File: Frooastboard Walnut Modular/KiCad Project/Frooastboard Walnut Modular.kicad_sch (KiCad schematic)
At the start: 88 parts, among them J1 SW Interface, J2 Conn_01x16, J3 Conn_01x06, J4 Conn_01x06, J5 Conn_01x10, J6 Conn_01x12, J7 Conn_01x04, U1 RP2040, U2 SPX3819M5-L-3-3, U3 W25Q32JVZP, U4 nRF8001, U5 IS31FL3733-QF, U6 FS312F-G, U7 FS8205, U8 IP2312, Y1 32.768kHz, Y2 16MHz, Y3 12MHz

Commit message: stuff
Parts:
- removed BT1: Battery_Cell, TestPoint:TestPoint_2Pads_Pitch5.08mm_Drill1.3mm, symbol Device:Battery_Cell
- removed C1, C2, C4: 100n, Capacitor_SMD:C_0402_1005Metric, symbol Device:C_Small
- removed C10, C11: 12p, Capacitor_SMD:C_0402_1005Metric, symbol Device:C_Small
- removed C12: 1.8p, Capacitor_SMD:C_0402_1005Metric, symbol Device:C_Small
- removed C13: 1.2p, Capacitor_SMD:C_0402_1005Metric, symbol Device:C_Small
- removed C29: 10n, Capacitor_SMD:C_0805_2012Metric, symbol Device:C_Small
- removed C3: 1n, Capacitor_SMD:C_0402_1005Metric, symbol Device:C_Small
- removed C30, C36: 22u, Capacitor_SMD:C_0805_2012Metric, symbol Device:C
- removed C31: 10u, Capacitor_SMD:C_0805_2012Metric, symbol Device:C_Small
- removed C32: 100n, Capacitor_SMD:C_0805_2012Metric, symbol Device:C_Small
- removed C37: 10u, Capacitor_SMD:C_0805_2012Metric, symbol Device:C
- removed C5: 33n, Capacitor_SMD:C_0402_1005Metric, symbol Device:C_Small
- removed C6, C7: 15p, Capacitor_SMD:C_0402_1005Metric, symbol Device:C_Small
- removed C8: 2.2n, Capacitor_SMD:C_0402_1005Metric, symbol Device:C_Small
- removed C9: Not Mounted, Capacitor_SMD:C_0402_1005Metric, symbol Device:C_Small
- removed D1: GREEN, LED_SMD:LED_0805_2012Metric, symbol Device:LED
- removed D2: RED, LED_SMD:LED_0805_2012Metric, symbol Device:LED
- removed L1: 5.6nH, Inductor_SMD:L_0402_1005Metric, symbol Device:L_Small
- removed L2: 8.2nH, Inductor_SMD:L_0402_1005Metric, symbol Device:L_Small
- removed L3: 3.9nH, Inductor_SMD:L_0402_1005Metric, symbol Device:L_Small
- removed L4: 1uH, Inductor_SMD:L_6.3x6.3_H3, symbol Device:L
- removed R1: 10k, Resistor_SMD:R_0805_2012Metric, symbol Device:R_Small
- removed R10: 2k, Resistor_SMD:R_0805_2012Metric, symbol Device:R
- removed R12: 0k5, Resistor_SMD:R_0805_2012Metric, symbol Device:R
- removed R13, R14: 1M, Resistor_SMD:R_0805_2012Metric, symbol Device:R_Small
- removed R15, R16: 0k1, Resistor_SMD:R_0805_2012Metric, symbol Device:R
- removed R17, R20: NC, Resistor_SMD:R_0805_2012Metric, symbol Device:R
- removed R18: 51k, Resistor_SMD:R_0805_2012Metric, symbol Device:R
- removed R19: 1k, Resistor_SMD:R_0805_2012Metric, symbol Device:R
- removed R2: 22k, Resistor_SMD:R_0805_2012Metric, symbol Device:R_Small
- removed TP1: NRF_TXD, TestPoint:TestPoint_Pad_D1.5mm, symbol Connector:TestPoint
- removed TP2: NRF_RXD, TestPoint:TestPoint_Pad_D1.5mm, symbol Connector:TestPoint
- removed TP3: NRF_RESET, TestPoint:TestPoint_Pad_D1.5mm, symbol Connector:TestPoint
- removed TP4: NRF_IREF, TestPoint:TestPoint_Pad_D1.5mm, symbol Connector:TestPoint
- removed U2: SPX3819M5-L-3-3, Package_TO_SOT_SMD:SOT-23-5, symbol Regulator_Linear:SPX3819M5-L-3-3
- removed U4: nRF8001, Package_DFN_QFN:QFN-32-1EP_5x5mm_P0.5mm_EP3.45x3.45mm, symbol RF_Bluetooth:nRF8001
- removed U6: FS312F-G, Package_TO_SOT_SMD:SOT-23-6, symbol Frooastboard Symbols:FS312F-G
- removed U7: FS8205, Package_TO_SOT_SMD:SOT-23-6, symbol Frooastboard Symbols:FS8205
- removed U8: IP2312, Package_SO:SOIC-8-1EP_3.9x4.9mm_P1.27mm_EP2.41x3.3mm, symbol Frooastboard Symbols:IP2312
- removed Y1: 32.768kHz, Crystal:Crystal_SMD_EuroQuartz_EQ161-2Pin_3.2x1.5mm, symbol Device:Crystal_Small
- removed Y2: 16MHz, Crystal:Crystal_SMD_3225-4Pin_3.2x2.5mm, symbol Device:Crystal_GND24_Small
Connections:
- no-connect marks 6 -> 3
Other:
- note removed: "NC for 2.1A"
- note removed: "NC for 4.2V"
- moved on the sheet: C28, C33, C34, C35, J2, J3, J4, R11, R6, R7, U5

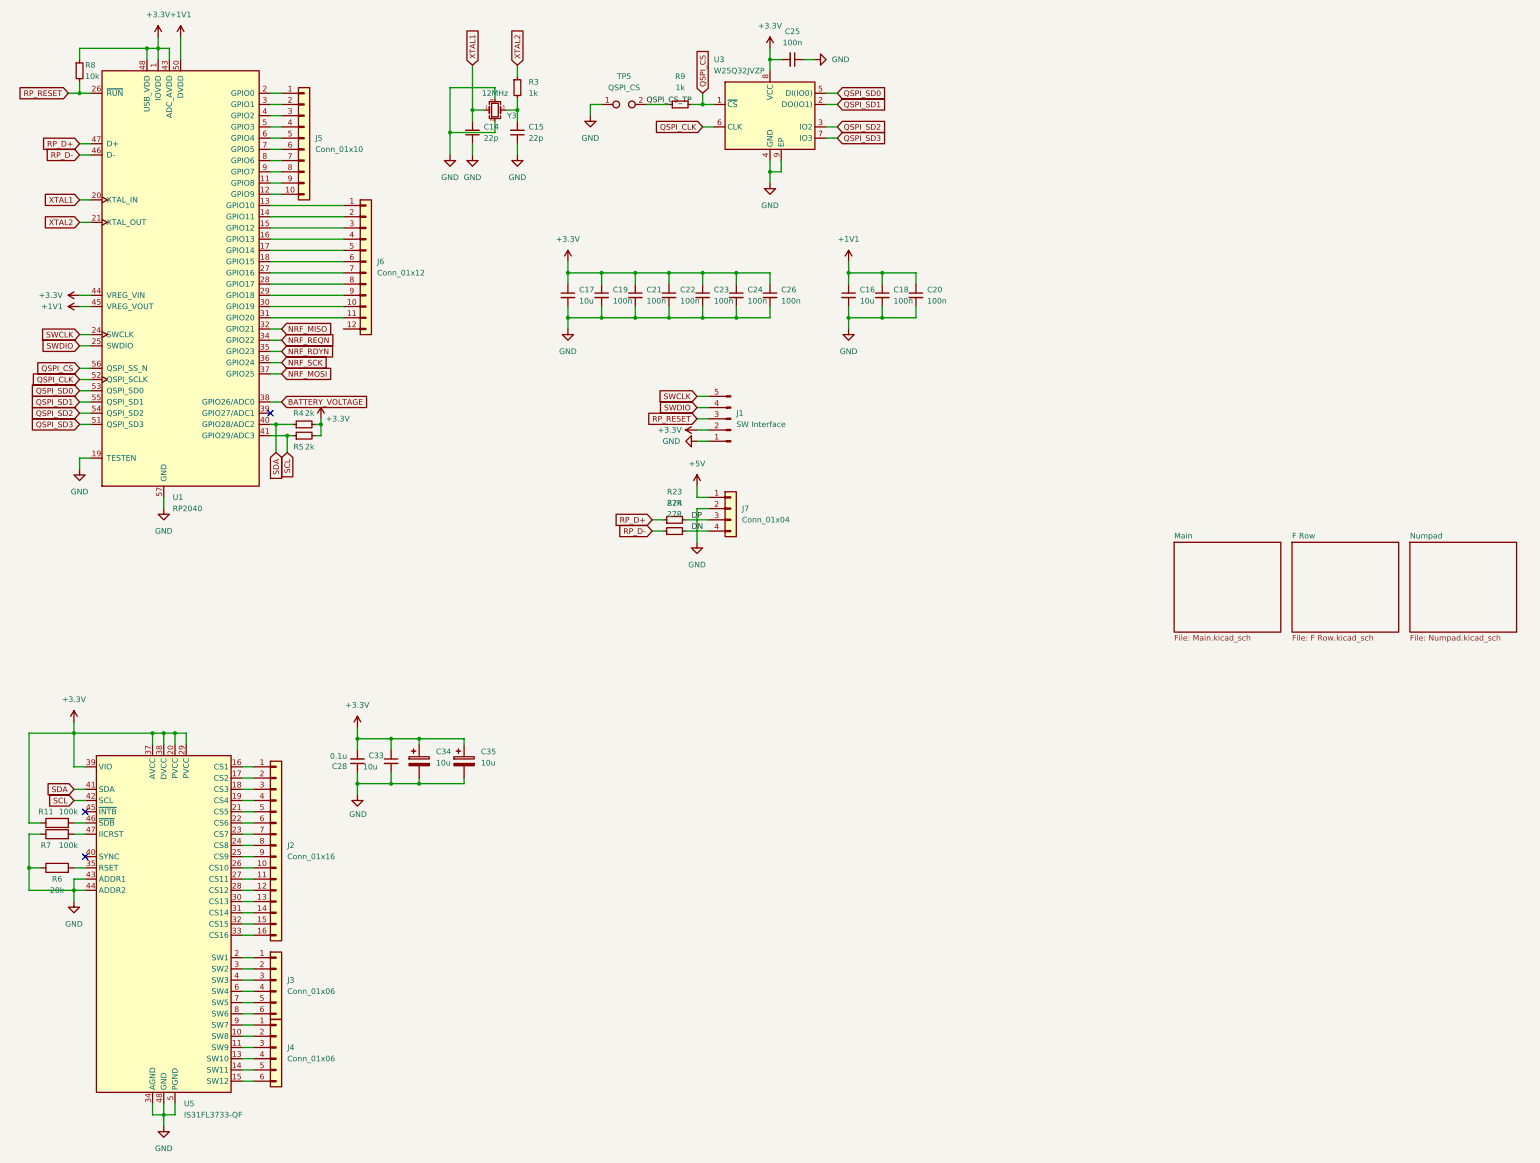
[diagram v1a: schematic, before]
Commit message: change some stuff maybe finally get started
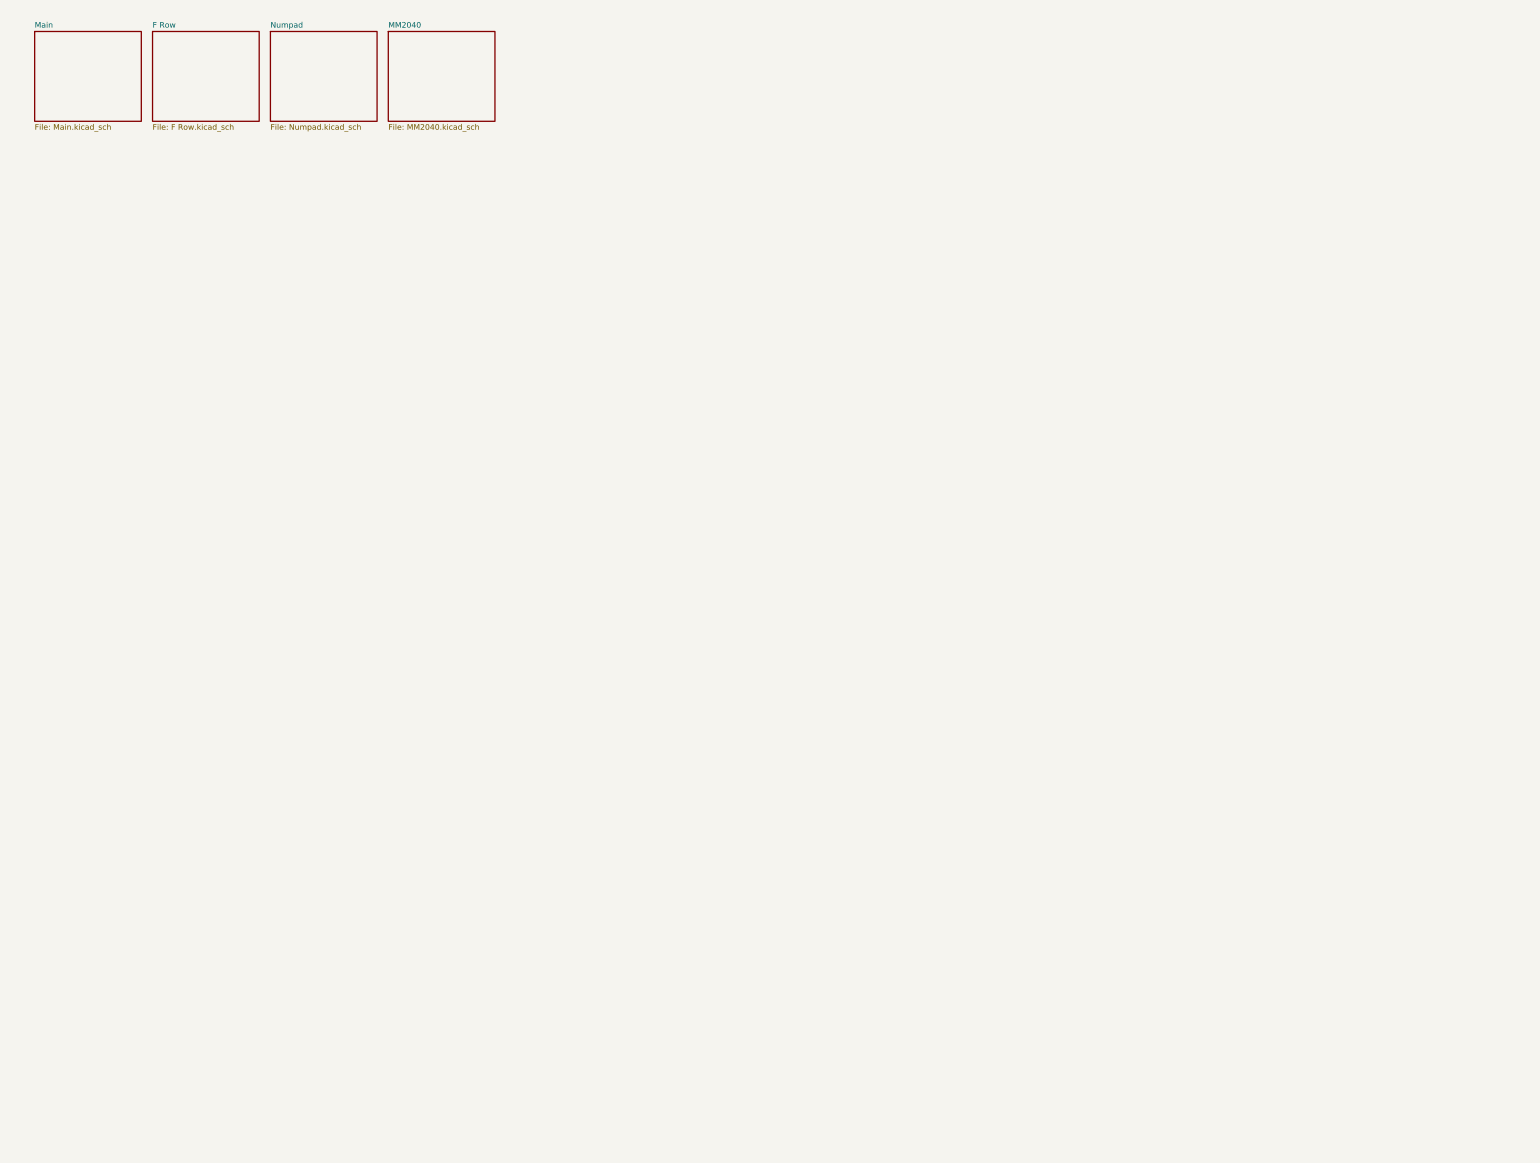
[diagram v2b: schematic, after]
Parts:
- removed C14, C15: 22p, Capacitor_SMD:C_0805_2012Metric, symbol Device:C_Small
- removed C16, C17, C33: 10u, Capacitor_SMD:C_0805_2012Metric, symbol Device:C_Small
- removed C18, C19, C20, C21, C22, C23, C24, C25, C26: 100n, Capacitor_SMD:C_0805_2012Metric, symbol Device:C_Small
- removed C28: 0.1u, Capacitor_SMD:C_0805_2012Metric, symbol Device:C_Small
- removed C34, C35: 10u, Capacitor_Tantalum_SMD:CP_EIA-2012-15_AVX-P, symbol Device:C_Polarized
- removed J1: SW Interface, Connector_PinHeader_1.27mm:PinHeader_1x05_P1.27mm_Vertical, symbol Connector:Conn_01x05_Male
- removed J2: Conn_01x16, Frooastboard Footprints:PinHeader_1x16_P1.27mm_Vertical, symbol Connector_Generic:Conn_01x16
- removed J3, J4: Conn_01x06, Frooastboard Footprints:PinHeader_1x06_P1.27mm_Vertical, symbol Connector_Generic:Conn_01x06
- removed J5: Conn_01x10, Frooastboard Footprints:PinHeader_1x10_P1.27mm_Vertical, symbol Connector_Generic:Conn_01x10
- removed J6: Conn_01x12, Frooastboard Footprints:PinHeader_1x12_P1.27mm_Vertical, symbol Connector_Generic:Conn_01x12
- removed J7: Conn_01x04, Frooastboard Footprints:PinHeader_1x04_P1.27mm_Vertical, symbol Connector_Generic:Conn_01x04
- removed R11, R7: 100k, Resistor_SMD:R_0805_2012Metric, symbol Device:R
- removed R23, R24: 27R, Resistor_SMD:R_0805_2012Metric, symbol Device:R_Small
- removed R3, R9: 1k, Resistor_SMD:R_0805_2012Metric, symbol Device:R_Small
- removed R4, R5: 2k, Resistor_SMD:R_0805_2012Metric, symbol Device:R_Small
- removed R6: 20k, Resistor_SMD:R_0805_2012Metric, symbol Device:R
- removed R8: 10k, Resistor_SMD:R_0805_2012Metric, symbol Device:R_Small
- removed TP5: QSPI_CS, Connector_PinHeader_1.27mm:PinHeader_1x02_P1.27mm_Vertical, symbol Connector:TestPoint_2Pole
- removed U1: RP2040, Frooastboard Footprints:RP2040-QFN-56, symbol Frooastboard Symbols:RP2040
- removed U3: W25Q32JVZP, Package_SON:WSON-8-1EP_6x5mm_P1.27mm_EP3.4x4.3mm, symbol Memory_Flash:W25Q32JVZP
- removed U5: IS31FL3733-QF, Package_DFN_QFN:QFN-48-1EP_6x6mm_P0.4mm_EP4.2x4.2mm, symbol Driver_LED:IS31FL3733-QF
- removed Y3: 12MHz, Crystal:Crystal_SMD_3225-4Pin_3.2x2.5mm, symbol Device:Crystal_GND24_Small
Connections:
- no-connect marks 3 -> 0
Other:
- added sheet MM2040 (MM2040.kicad_sch)
